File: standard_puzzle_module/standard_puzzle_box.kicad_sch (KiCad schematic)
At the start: 1 part, among them U1 ESP32-C3-DevKitM-1

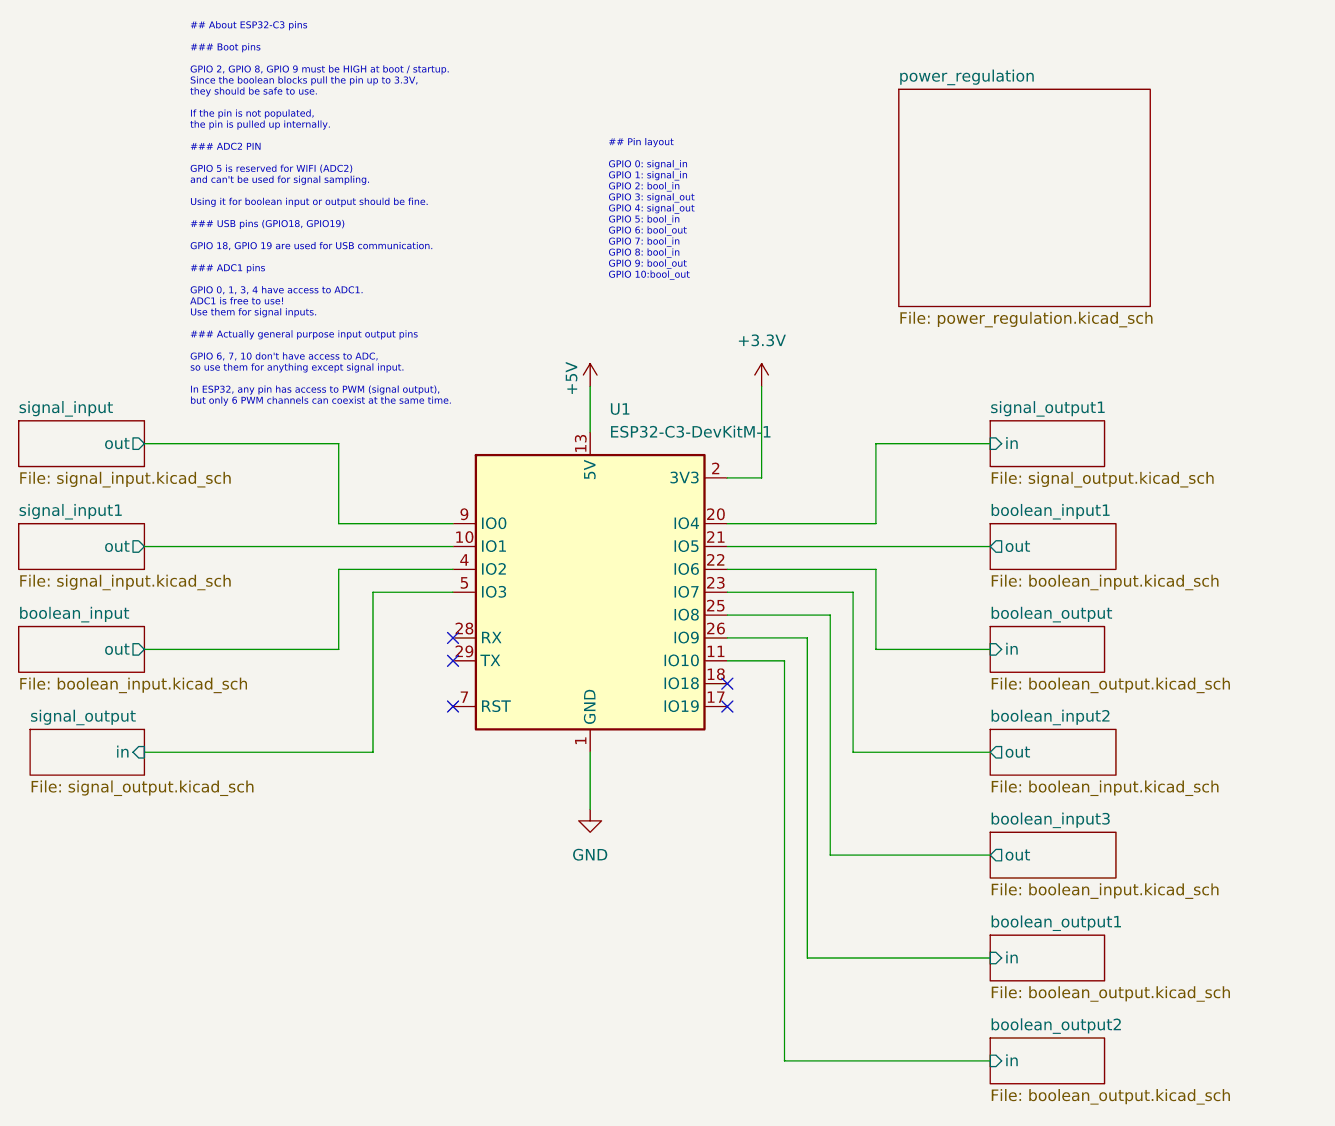
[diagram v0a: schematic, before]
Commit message: feat: salvaging stuff after lossy crash
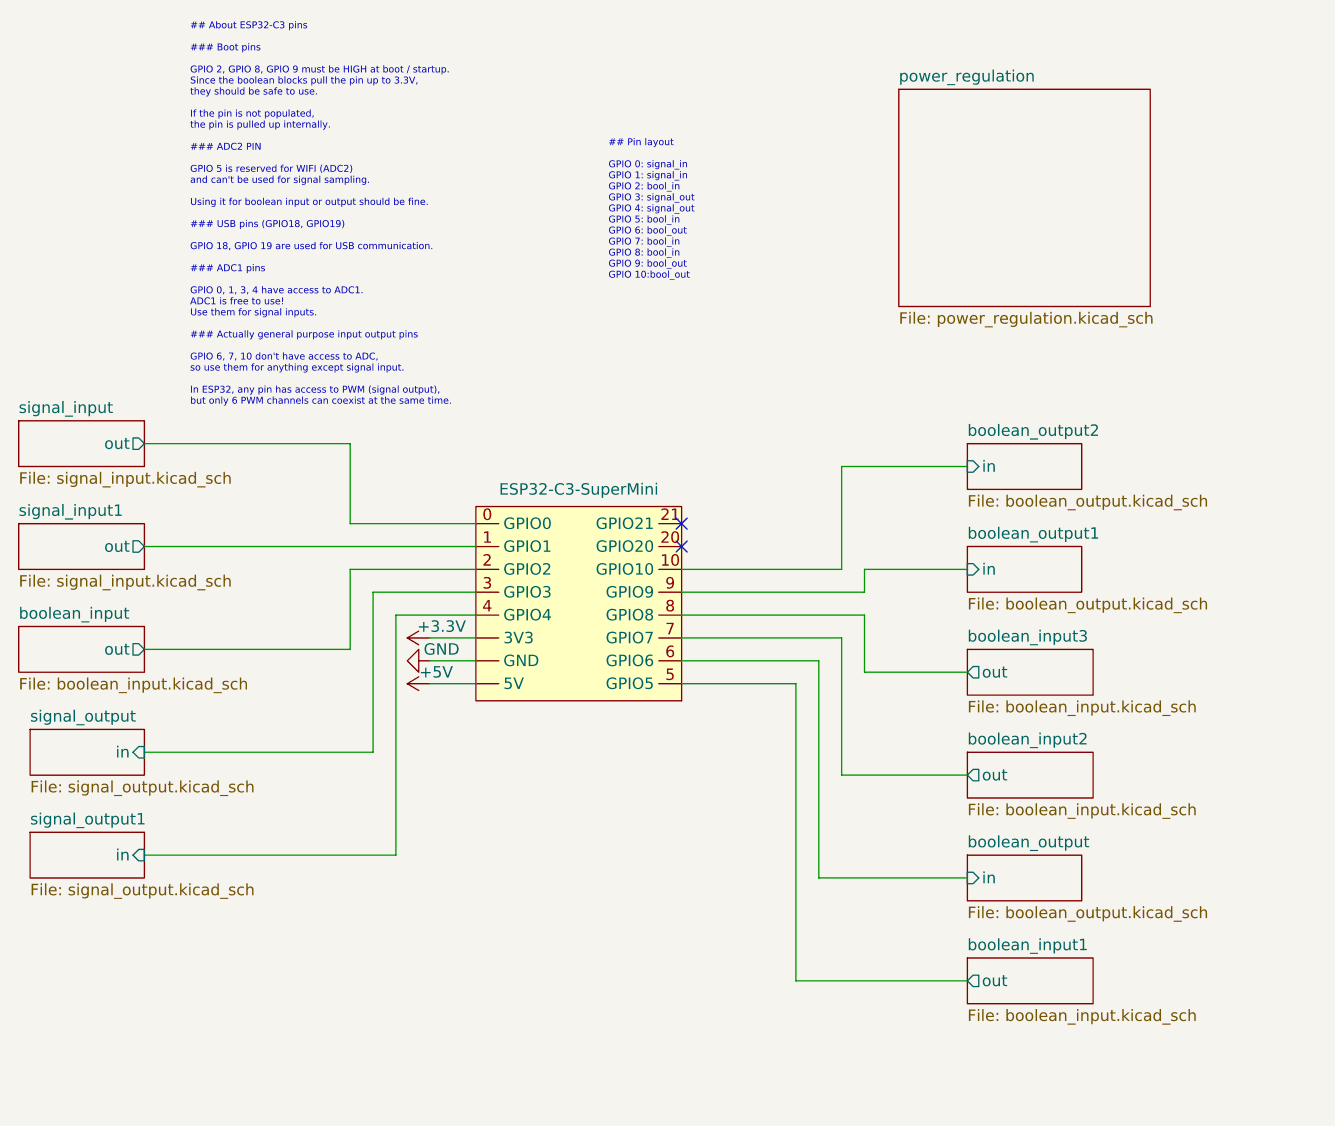
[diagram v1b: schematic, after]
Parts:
- removed U1: ESP32-C3-DevKitM-1, RF_Module:ESP32-C3-DevKitM-1, symbol RF_Module:ESP32-C3-DevKitM-1
- added U2: ESP32-C3-SuperMini, ESP32C3-SuperMini:ESP32-C3-SuperMini, symbol ESP32-C3-SuperMini:ESP32-C3-SuperMini
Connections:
- net +3.3V: now also U2. (3V3)
- net +5V: now also U2. (3V3)
- net GND: now also U2. (3V3)
- net boolean_input/out: now also U2.2 (GPIO2)
- net boolean_input1/out: now also U2.5 (GPIO5)
- net boolean_input2/out: now also U2.7 (GPIO7)
- net boolean_input3/out: now also U2.8 (GPIO8)
- net boolean_output/in: now also U2.6 (GPIO6)
- net boolean_output1/in: now also U2.9 (GPIO9)
- net boolean_output2/in: now also U2.10 (GPIO10)
- net signal_input/out: now also U2.0 (GPIO0)
- net signal_input1/out: now also U2.1 (GPIO1)
- net signal_output/in: now also U2.3 (GPIO3)
- net signal_output1/in: now also U2.4 (GPIO4)
- no-connect marks 5 -> 2
